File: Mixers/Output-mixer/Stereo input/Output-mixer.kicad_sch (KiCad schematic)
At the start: 123 parts, among them J1 In, J10 In, J11 In, J12 In, J13 Power Input, J14 Conn_01x04_Female, J15 Conn_01x02_Male, J16 Conn_01x04_Male, J17 Conn_01x02_Female, J18 OutR, J19 OutL, J2 In, J20 Jack 3.5 Out, J21 Jack 3.5 Out, J22 OutL, J23 OutR, J3 In, J4 In, J5 In, J6 In, J7 In, J8 In, J9 In, SW1 Mute, SW2 Mute, SW3 Mute, SW4 Mute, SW5 Mute, SW6 Mute, U1 TL072, U2 TL072, U3 TL072, U4 TL072, U5 TL072, U6 TL072, U7 TL072

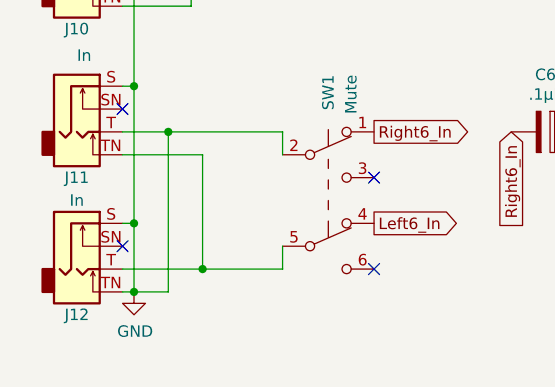
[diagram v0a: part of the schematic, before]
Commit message: finish updating PCB
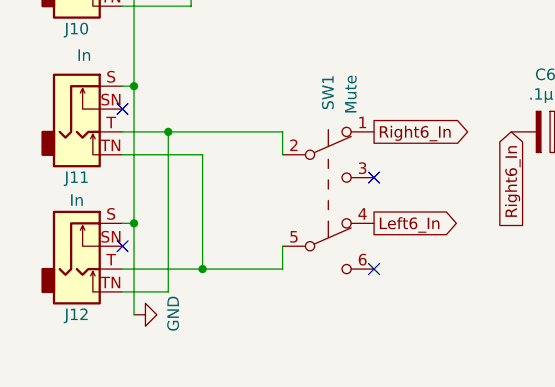
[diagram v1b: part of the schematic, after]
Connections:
- net GND: no longer J11.T, J12.TN, SW1.2 (B)
- new net: J11.T, J12.TN, SW1.2 (B)
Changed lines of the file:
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@@
   (junction (at 82.55 86.36) (diameter 0) (color 0 0 0 0)
   )
-  (junction (at 22.86 193.04) (diameter 0) (color 0 0 0 0)
-  )
   (junction (at 260.35 93.98) (diameter 0) (color 0 0 0 0)
   )
@@
     (stroke (width 0) (type default) (color 0 0 0 0))
   )
-  (wire (pts (xy 21.59 193.04) (xy 22.86 193.04))
-    (stroke (width 0) (type default) (color 0 0 0 0))
-  )
   (wire (pts (xy 165.1 45.72) (xy 165.1 43.18))
     (stroke (width 0) (type default) (color 0 0 0 0))
@@
     (stroke (width 0) (type default) (color 0 0 0 0))
   )
-  (wire (pts (xy 22.86 185.42) (xy 22.86 193.04))
+  (wire (pts (xy 22.86 185.42) (xy 22.86 195.58))
     (stroke (width 0) (type default) (color 0 0 0 0))
   )
@@
     (stroke (width 0) (type default) (color 0 0 0 0))
   )
-  (wire (pts (xy 22.86 193.04) (xy 26.67 193.04))
+  (wire (pts (xy 21.59 193.04) (xy 26.67 193.04))
     (stroke (width 0) (type default) (color 0 0 0 0))
   )
@@
       (effects (font (size 1.27 1.27)) hide)
     )
-    (pin "1")
-    (pin "2")
-    (pin "3")
-    (pin "5")
-    (pin "6")
-    (pin "7")
     (pin "4")
     (pin "8")
@@
     (pin "2")
     (pin "3")
-    (pin "4")
-    (pin "5")
-    (pin "6")
   )
   (symbol (lib_id "Connector:AudioJack2_Switch") (at 16.51 158.75 0) (unit 1)
@@
     (pin "2")
     (pin "3")
-    (pin "4")
-    (pin "5")
-    (pin "6")
   )
   (symbol (lib_id "power:+12V") (at 247.65 25.4 0) (unit 1)
@@
     (pin "2")
     (pin "3")
-    (pin "4")
-    (pin "5")
-    (pin "6")
   )
   (symbol (lib_id "Device:R") (at 93.98 35.56 270) (unit 1)
@@
       (effects (font (size 1.27 1.27)) hide)
     )
-    (pin "1")
-    (pin "2")
-    (pin "3")
-    (pin "5")
-    (pin "6")
-    (pin "7")
     (pin "4")
     (pin "8")
@@
     (pin "2")
     (pin "3")
-    (pin "5")
-    (pin "6")
-    (pin "7")
-    (pin "4")
-    (pin "8")
   )
   (symbol (lib_id "Device:C_Small") (at 212.09 45.72 0) (unit 1)
@@
     (pin "2")
     (pin "3")
-    (pin "5")
-    (pin "6")
-    (pin "7")
-    (pin "4")
-    (pin "8")
   )
   (symbol (lib_id "Device:C_Small") (at 181.61 33.02 0) (unit 1)
@@
     (pin "2")
     (pin "3")
-    (pin "4")
-    (pin "5")
-    (pin "6")
   )
   (symbol (lib_id "Device:R") (at 135.89 185.42 270) (unit 1)
@@
     (pin "2")
     (pin "3")
-    (pin "5")
-    (pin "6")
-    (pin "7")
-    (pin "4")
-    (pin "8")
   )
   (symbol (lib_id "Device:CP") (at 214.63 72.39 90) (unit 1)
@@
       (effects (font (size 1.27 1.27)) hide)
     )
-    (pin "1")
-    (pin "2")
-    (pin "3")
     (pin "4")
     (pin "5")
@@
     (pin "2")
     (pin "3")
-    (pin "4")
-    (pin "5")
-    (pin "6")
   )
   (symbol (lib_id "Switch:SW_Push_DPDT") (at 46.99 62.23 0) (unit 1)
@@
     (pin "2")
     (pin "3")
-    (pin "4")
-    (pin "5")
-    (pin "6")
   )
   (symbol (lib_id "Amplifier_Operational:TL072") (at 95.25 25.4 0) (unit 1)
@@
     (pin "2")
     (pin "3")
-    (pin "5")
-    (pin "6")
-    (pin "7")
-    (pin "4")
-    (pin "8")
   )
   (symbol (lib_id "Device:R") (at 194.31 115.57 270) (unit 1)
@@
     (pin "2")
     (pin "3")
-    (pin "5")
-    (pin "6")
-    (pin "7")
-    (pin "4")
-    (pin "8")
   )
   (symbol (lib_id "Device:R") (at 135.89 83.82 90) (unit 1)
@@
     (pin "2")
   )
-  (symbol (lib_id "power:GND") (at 22.86 193.04 0) (unit 1)
+  (symbol (lib_id "power:GND") (at 22.86 195.58 90) (unit 1)
     (in_bom yes) (on_board yes)
-    (property "Reference" "#PWR01" (id 0) (at 22.86 199.39 0)
+    (property "Reference" "#PWR01" (id 0) (at 29.21 195.58 0)
       (effects (font (size 1.27 1.27)) hide)
     )
-    (property "Value" "GND" (id 1) (at 22.987 197.4342 0))
-    (property "Footprint" "" (id 2) (at 22.86 193.04 0)
+    (property "Value" "GND" (id 1) (at 27.2542 195.453 0))
+    (property "Footprint" "" (id 2) (at 22.86 195.58 0)
       (effects (font (size 1.27 1.27)) hide)
     )
-    (property "Datasheet" "" (id 3) (at 22.86 193.04 0)
+    (property "Datasheet" "" (id 3) (at 22.86 195.58 0)
       (effects (font (size 1.27 1.27)) hide)
     )
@@
       (effects (font (size 1.27 1.27)) hide)
     )
-    (pin "1")
-    (pin "2")
-    (pin "3")
-    (pin "5")
-    (pin "6")
-    (pin "7")
     (pin "4")
     (pin "8")
@@
     (pin "2")
     (pin "3")
-    (pin "5")
-    (pin "6")
-    (pin "7")
-    (pin "4")
-    (pin "8")
   )
   (symbol (lib_id "Device:R") (at 118.11 55.88 90) (unit 1)
@@
       (effects (font (size 1.27 1.27)) hide)
     )
-    (pin "1")
-    (pin "2")
-    (pin "3")
     (pin "5")
     (pin "6")
     (pin "7")
-    (pin "4")
-    (pin "8")
   )
   (symbol (lib_id "Device:R") (at 77.47 116.84 270) (unit 1)
@@
       (effects (font (size 1.27 1.27)) hide)
     )
-    (pin "1")
-    (pin "2")
-    (pin "3")
-    (pin "5")
-    (pin "6")
-    (pin "7")
     (pin "4")
     (pin "8")
@@
     (pin "2")
     (pin "3")
-    (pin "4")
-    (pin "5")
-    (pin "6")
   )
   (symbol (lib_id "Device:C_Small") (at 191.77 45.72 0) (unit 1)
@@
     (pin "2")
     (pin "3")
-    (pin "5")
-    (pin "6")
-    (pin "7")
-    (pin "4")
-    (pin "8")
   )
   (symbol (lib_id "Device:C_Small") (at 181.61 45.72 0) (unit 1)
